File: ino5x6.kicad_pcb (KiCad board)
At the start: 2 copper layers, 62 parts, among them SW1 SW_Push, SW10 SW_Push, SW11 SW_Push, SW12 SW_Push, SW13 SW_Push, SW14 SW_Push, SW15 SW_Push, SW16 SW_Push, SW17 SW_Push, SW18 SW_Push, SW19 SW_Push, SW2 SW_Push, SW20 SW_Push, SW21 SW_Push, SW22 SW_Push, SW23 SW_Push, SW24 SW_Push, SW25 SW_Push, SW26 SW_Push, SW27 SW_Push, SW28 SW_Push, SW29 SW_Push, SW3 SW_Push, SW30 SW_Push, SW4 SW_Push, SW5 SW_Push, SW6 SW_Push, SW7 SW_Push, SW8 SW_Push, SW9 SW_Push, U1 ProMicro

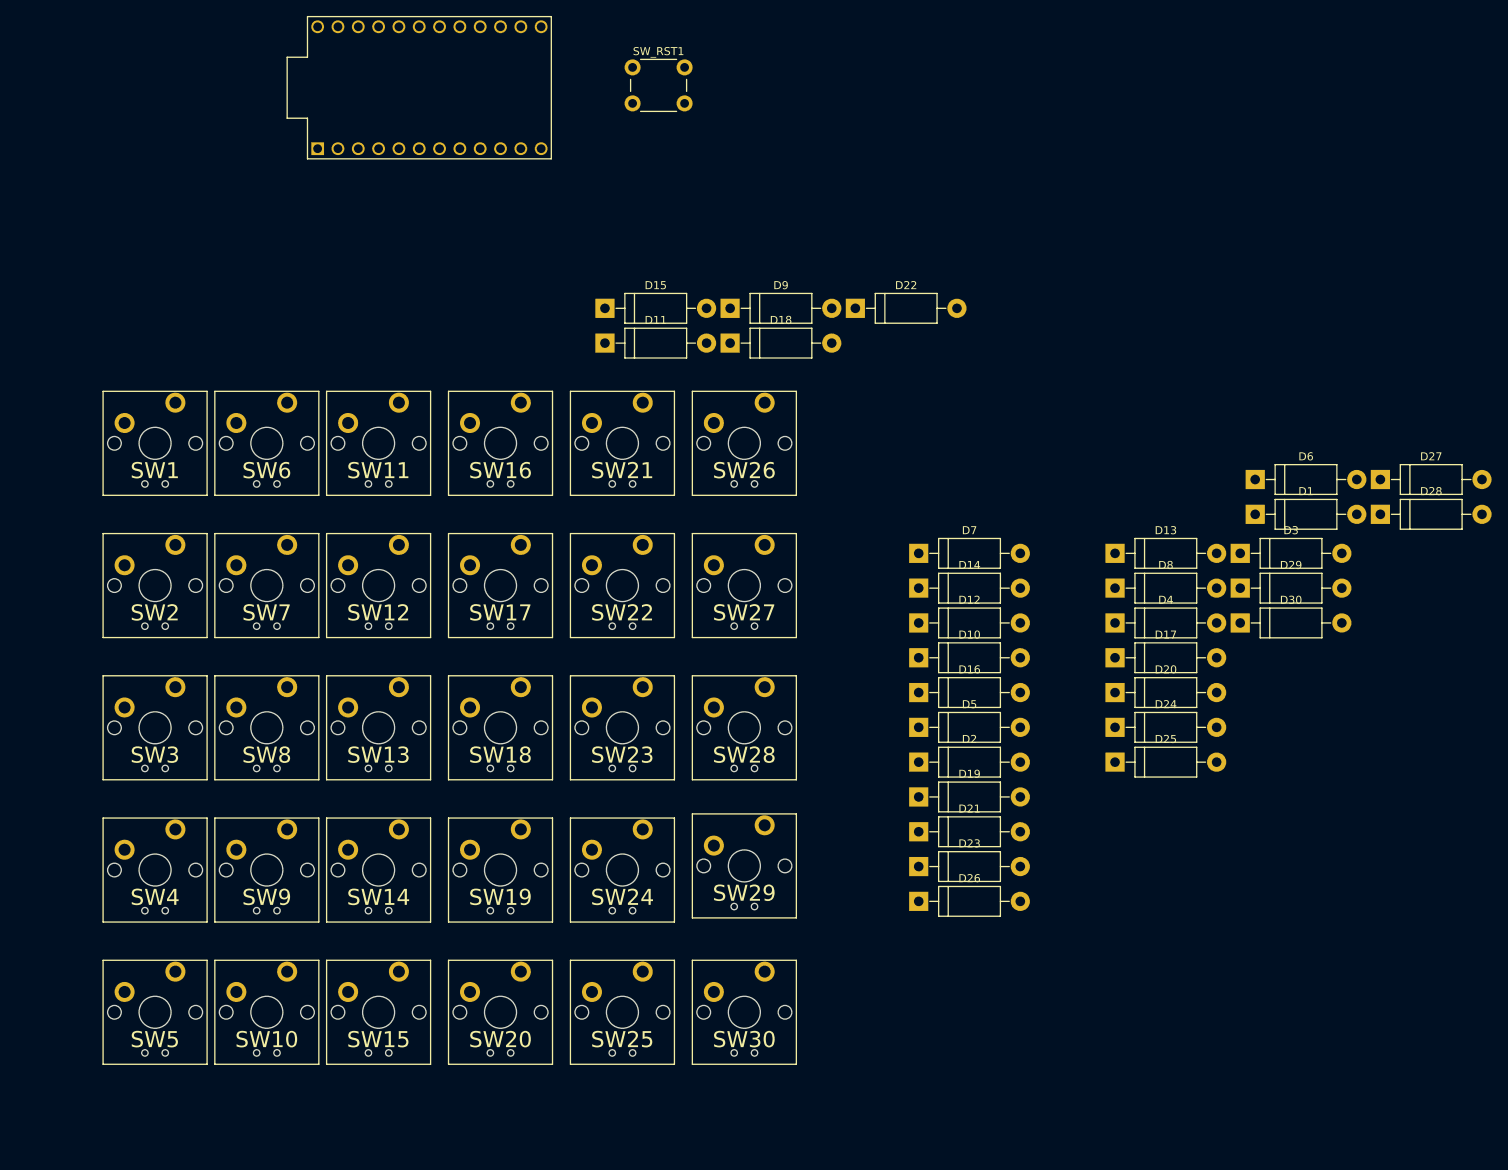
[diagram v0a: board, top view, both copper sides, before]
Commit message: 一応出来たがおかしい
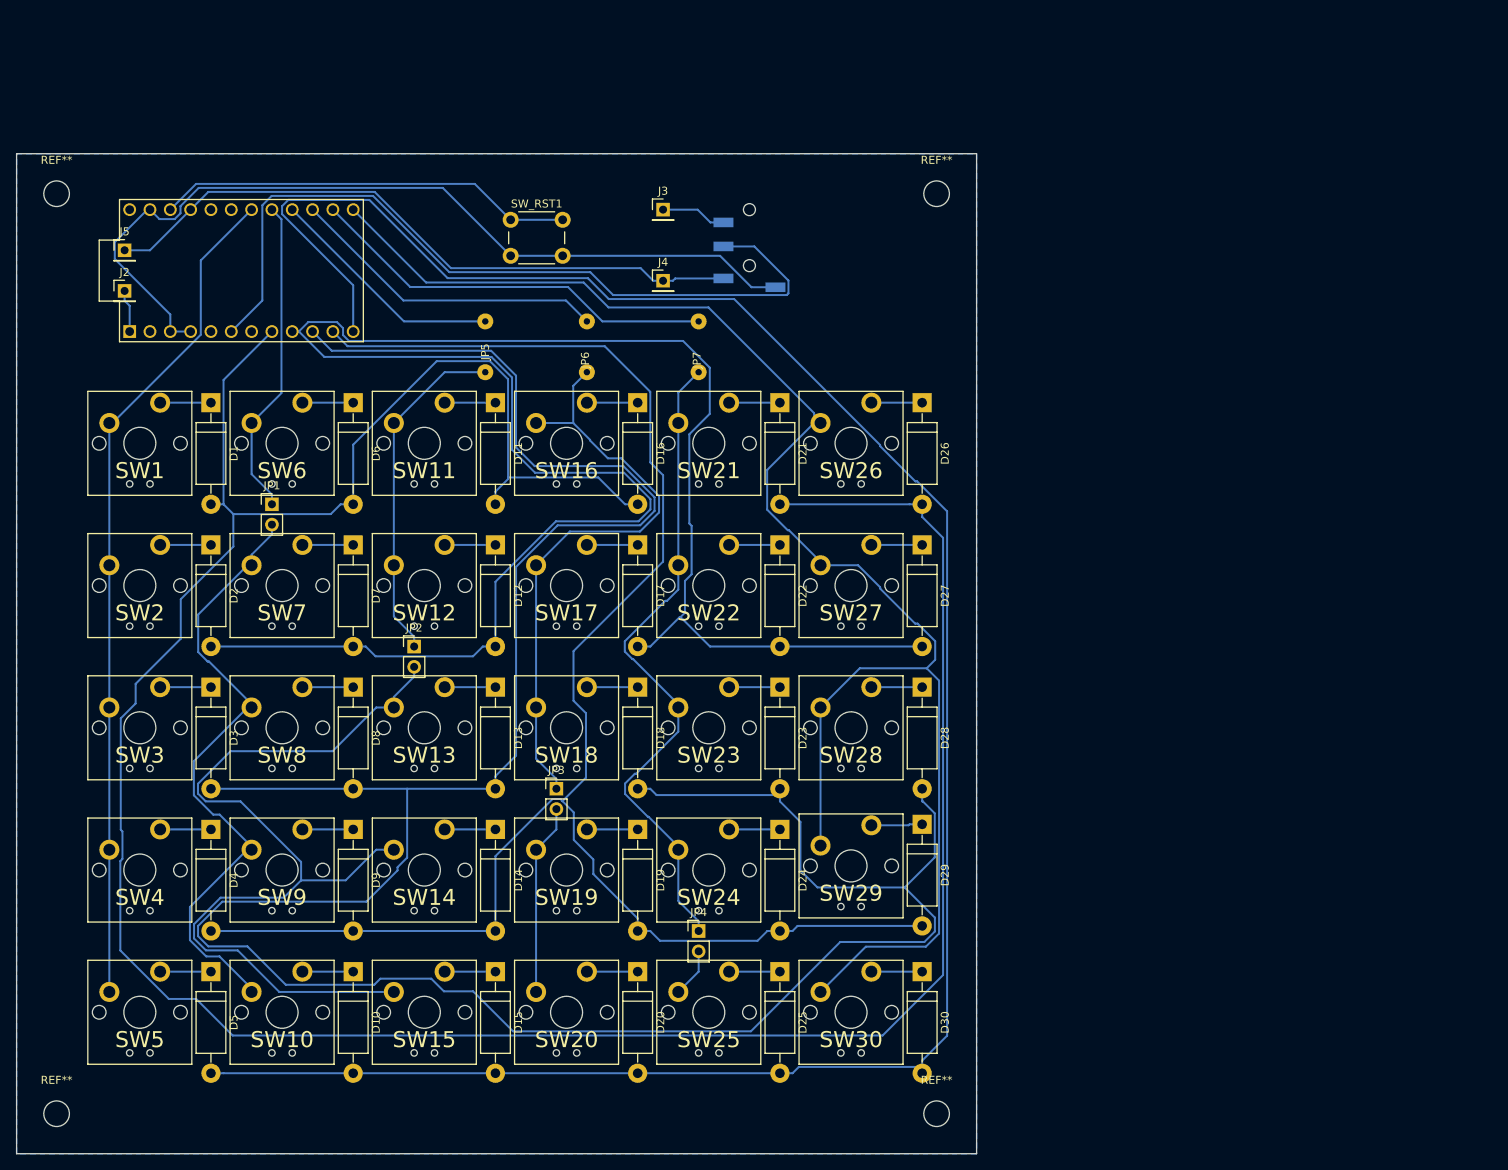
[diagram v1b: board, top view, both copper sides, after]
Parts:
- added J1: Conn_01x04_Male, Connectors:PJ320D_3.5mm_Jack, B.Cu at (141.6, 51.8)
- added J2: Conn_01x01_Male, Pin_Headers:Pin_Header_Straight_1x01_Pitch2.54mm, F.Cu at (63.5, 57.1)
- added J3: Conn_01x01_Male, Pin_Headers:Pin_Header_Straight_1x01_Pitch2.54mm, F.Cu at (130.8, 47.0)
- added J4: Conn_01x01_Male, Pin_Headers:Pin_Header_Straight_1x01_Pitch2.54mm, F.Cu at (130.8, 55.9)
- added J5: Conn_01x01_Male, Pin_Headers:Pin_Header_Straight_1x01_Pitch2.54mm, F.Cu at (63.5, 52.1)
- added JP1: Jumper_2_Bridged, Pin_Headers:Pin_Header_Straight_1x02_Pitch2.54mm, F.Cu at (81.9, 83.8)
- added JP2: Jumper_2_Bridged, Pin_Headers:Pin_Header_Straight_1x02_Pitch2.54mm, F.Cu at (99.7, 101.6)
- added JP3: Jumper_2_Bridged, Pin_Headers:Pin_Header_Straight_1x02_Pitch2.54mm, F.Cu at (117.5, 119.4)
- added JP4: Jumper_2_Bridged, Pin_Headers:Pin_Header_Straight_1x02_Pitch2.54mm, F.Cu at (135.3, 137.2)
- added JP5: Jumper_2_Bridged, Wire_Connections_Bridges:WireConnection_0.80mmDrill, F.Cu at (108.6, 61.0)
- added JP6: Jumper_2_Bridged, Wire_Connections_Bridges:WireConnection_0.80mmDrill, F.Cu at (121.3, 61.0)
- added JP7: Jumper_2_Bridged, Wire_Connections_Bridges:WireConnection_0.80mmDrill, F.Cu at (135.3, 61.0)
- added REF**: MountingHole_3.2mm_M3, Mounting_Holes:MountingHole_3.2mm_M3, F.Cu at (165.0, 45.0)
- added REF**: MountingHole_3.2mm_M3, Mounting_Holes:MountingHole_3.2mm_M3, F.Cu at (165.0, 160.0)
- added REF**: MountingHole_3.2mm_M3, Mounting_Holes:MountingHole_3.2mm_M3, F.Cu at (55.0, 160.0)
- added REF**: MountingHole_3.2mm_M3, Mounting_Holes:MountingHole_3.2mm_M3, F.Cu at (55.0, 45.0)
- moved D1 131.3 mm to (74.3, 71.1), turned to 270 degrees
- moved D3 129.7 mm to (74.3, 106.7), turned to 270 degrees
- moved D4 115.9 mm to (74.3, 124.5), turned to 270 degrees
- moved D6 113.2 mm to (92.1, 71.1), turned to 270 degrees
- moved D8 96.0 mm to (92.1, 106.7), turned to 270 degrees
- moved D5 93.6 mm to (74.3, 142.2), turned to 270 degrees
- moved D2 92.5 mm to (74.3, 88.9), turned to 270 degrees
- moved D15 84.0 mm to (109.9, 142.2), turned to 270 degrees
- moved D10 80.8 mm to (92.1, 142.2), turned to 270 degrees
- moved D9 80.4 mm to (92.1, 124.5), turned to 270 degrees
- moved D13 79.2 mm to (109.9, 106.7), turned to 270 degrees
- moved D7 70.7 mm to (92.1, 88.9), turned to 270 degrees
- moved D20 69.1 mm to (127.6, 142.2), turned to 270 degrees
- moved D26 62.3 mm to (163.2, 71.1), turned to 270 degrees
- moved D17 61.3 mm to (127.6, 88.9), turned to 270 degrees
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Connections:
- SW10 pad 1: /col1 -> Net-(JP1-Pad2)
- SW11 pad 1: /col2 -> Net-(JP2-Pad1)
- SW12 pad 1: /col2 -> Net-(JP2-Pad1)
- SW13 pad 1: /col2 -> Net-(JP2-Pad2)
- SW14 pad 1: /col2 -> Net-(JP2-Pad2)
- SW15 pad 1: /col2 -> Net-(JP2-Pad2)
- SW16 pad 1: /col3 -> Net-(JP3-Pad1)
- SW17 pad 1: /col3 -> Net-(JP3-Pad1)
- SW18 pad 1: /col3 -> Net-(JP3-Pad1)
- SW19 pad 1: /col3 -> Net-(JP3-Pad2)
- SW20 pad 1: /col3 -> Net-(JP3-Pad2)
- SW21 pad 1: /col4 -> Net-(JP4-Pad1)
- SW22 pad 1: /col4 -> Net-(JP4-Pad1)
- SW23 pad 1: /col4 -> Net-(JP4-Pad1)
- SW24 pad 1: /col4 -> Net-(JP4-Pad1)
- SW25 pad 1: /col4 -> Net-(JP4-Pad2)
- SW7 pad 1: /col1 -> Net-(JP1-Pad2)
- SW8 pad 1: /col1 -> Net-(JP1-Pad2)
- SW9 pad 1: /col1 -> Net-(JP1-Pad2)
- U1 pad 6: Net-(U1-Pad6) -> /sda
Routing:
- net /row0: track 0.00 -> 357.5 mm
- net /row2: track 0.00 -> 350.4 mm
- net /row4: track 0.00 -> 279.8 mm
- net /row1: track 0.00 -> 254.1 mm
- net /row3: track 0.00 -> 214.5 mm
- net /col5: track 0.00 -> 199.6 mm
- net Net-(JP2-Pad2): track 0.00 -> 112.9 mm
- net GND: track 0.00 -> 108.6 mm
- net /col0: track 0.00 -> 105.4 mm
- net /sda: track 0.00 -> 100.4 mm
- net Net-(JP4-Pad1): track 0.00 -> 83.3 mm
- net VCC: track 0.00 -> 82.6 mm
- net Net-(JP1-Pad2): track 0.00 -> 79.4 mm
- net Net-(JP3-Pad1): track 0.00 -> 75.4 mm
- net Net-(SW_RST1-Pad1): track 0.00 -> 52.2 mm
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- added copper zone on B.Cu, net GND
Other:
- board outline added: 120 x 125 mm
- net class Default: clearance 0.2 -> 0.25
- rule trace_clearance: 0.2 -> 0.25
